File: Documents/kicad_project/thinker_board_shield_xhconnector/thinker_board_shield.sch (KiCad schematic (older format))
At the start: 10 parts, among them J1 Jack-DC, J2 Thinker_board_S, U1 XH_S, U2 1PIN, U3 XH_4PIN, U4 2_pin

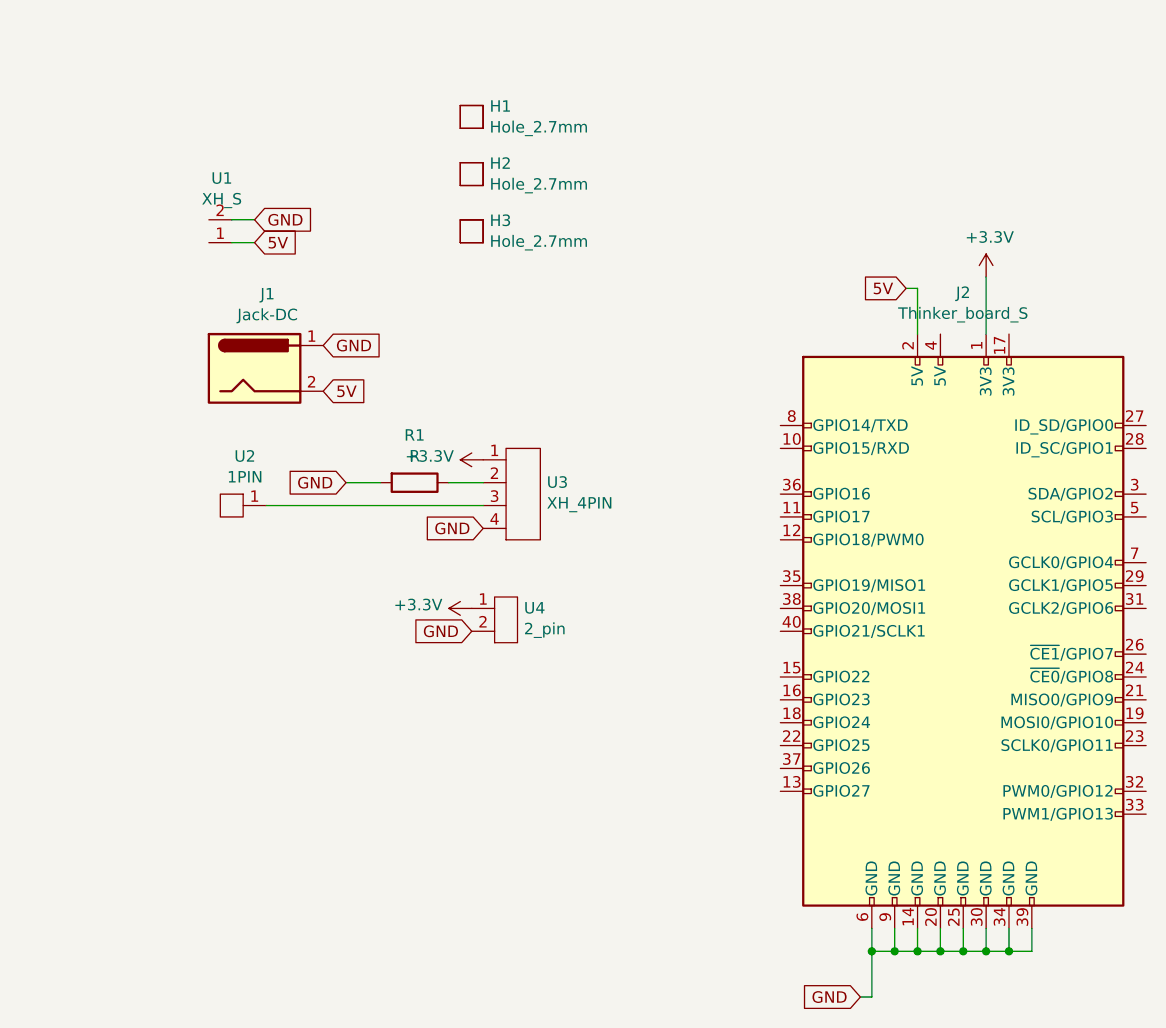
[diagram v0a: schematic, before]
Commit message: change to raspi
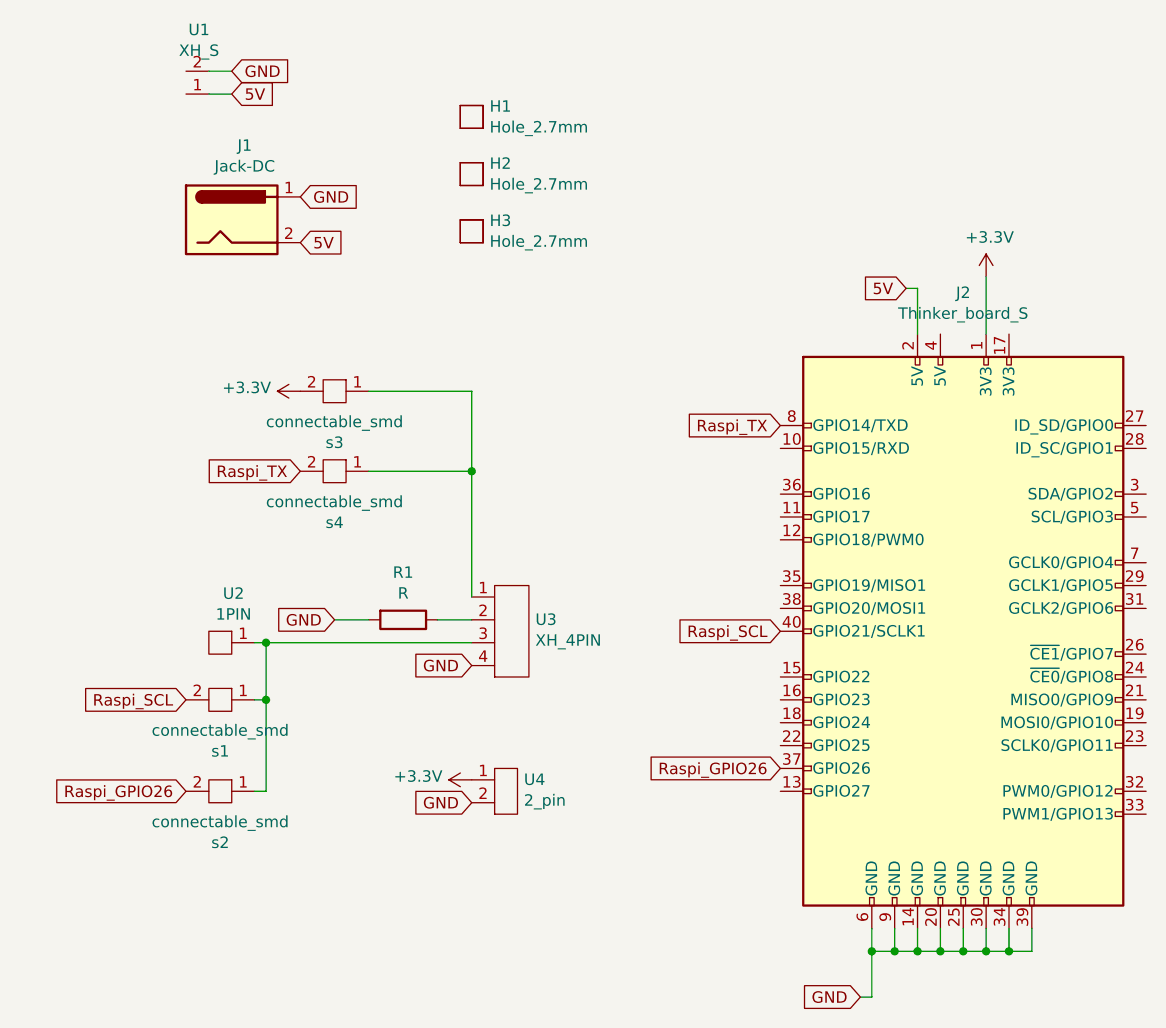
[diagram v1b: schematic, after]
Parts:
- added s1, s2, s3, s4: connectable_smd, hoshina_library:connectable_smd, symbol hoshina_library:connectable_smd
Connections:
- net +3V3: now also s3.2; no longer U3.1
- net Raspi_GPIO26: now reaches J2.37 (GPIO26)
- net Raspi_GPIO26: now also s2.2
- net Raspi_SCL: now reaches J2.40 (GPIO21/SCLK1)
- net Raspi_SCL: now also s1.2
- net Raspi_TX: now reaches J2.8 (GPIO14/TXD)
- net Raspi_TX: now also s4.2
- net at U2.1, U3.3: now also s1.1, s2.1
- new net: U3.1, s3.1, s4.1
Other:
- moved on the sheet: J1, R1, U1, U2, U3, U4
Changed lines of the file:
@@
 	1    0    0    -1
 $EndComp
-Text GLabel 1900 3450 2    50   Input ~ 0
+Text GLabel 1800 2800 2    50   Input ~ 0
 5V
-Text GLabel 1900 3250 2    50   Input ~ 0
+Text GLabel 1800 2600 2    50   Input ~ 0
 GND
 Text GLabel 4450 3000 0    50   Input ~ 0
@@
 Connection ~ 4900 5900
 Wire Wire Line
-	1500 2700 1600 2700
-Wire Wire Line
-	1600 2800 1500 2800
+	1400 2050 1500 2050
+Wire Wire Line
+	1500 2150 1400 2150
 $Comp
 L hoshina_library:XH_S U1
 U 1 1 5D710EE3
-P 1500 2700
-F 0 "U1" H 1543 2519 50  0000 C CNN
-F 1 "XH_S" H 1543 2610 50  0000 C CNN
-F 2 "hoshina_library:S2B-XH-A" H 1500 2600 50  0001 C CNN
-F 3 "" H 1500 2600 50  0001 C CNN
-	1    1500 2700
+P 1400 2050
+F 0 "U1" H 1443 1869 50  0000 C CNN
+F 1 "XH_S" H 1443 1960 50  0000 C CNN
+F 2 "hoshina_library:S2B-XH-A" H 1400 1950 50  0001 C CNN
+F 3 "" H 1400 1950 50  0001 C CNN
+	1    1400 2050
 	-1   0    0    1
 $EndComp
@@
 L hoshina_library:XH_4PIN U3
 U 1 1 5D76ADEE
-P 2600 3950
-F 0 "U3" H 2878 4051 50  0000 L CNN
-F 1 "XH_4PIN" H 2878 3960 50  0000 L CNN
-F 2 "hoshina_library:XH4PIN_S" H 2600 3750 50  0001 C CNN
-F 3 "" H 2600 3750 50  0001 C CNN
-	1    2600 3950
+P 2550 4550
+F 0 "U3" H 2828 4651 50  0000 L CNN
+F 1 "XH_4PIN" H 2828 4560 50  0000 L CNN
+F 2 "hoshina_library:XH4PIN_S" H 2550 4350 50  0001 C CNN
+F 3 "" H 2550 4350 50  0001 C CNN
+	1    2550 4550
 	1    0    0    -1
 $EndComp
@@
 L power:+3.3V #PWR0101
 U 1 1 5D76B7AA
-P 2600 3750
-F 0 "#PWR0101" H 2600 3600 50  0001 C CNN
-F 1 "+3.3V" V 2615 3878 50  0000 L CNN
-F 2 "" H 2600 3750 50  0001 C CNN
-F 3 "" H 2600 3750 50  0001 C CNN
-	1    2600 3750
+P 1800 3450
+F 0 "#PWR0101" H 1800 3300 50  0001 C CNN
+F 1 "+3.3V" V 1815 3578 50  0000 L CNN
+F 2 "" H 1800 3450 50  0001 C CNN
+F 3 "" H 1800 3450 50  0001 C CNN
+	1    1800 3450
 	0    -1   -1   0
 $EndComp
-Text GLabel 2000 3850 0    50   Input ~ 0
+Text GLabel 1950 4450 0    50   Input ~ 0
 GND
 $Comp
 L Device:R R1
 U 1 1 5D76C583
-P 2300 3850
-F 0 "R1" V 2093 3850 50  0000 C CNN
-F 1 "R" V 2184 3850 50  0000 C CNN
-F 2 "hoshina_library:register_0603" V 2230 3850 50  0001 C CNN
-F 3 "~" H 2300 3850 50  0001 C CNN
-	1    2300 3850
+P 2250 4450
+F 0 "R1" V 2043 4450 50  0000 C CNN
+F 1 "R" V 2134 4450 50  0000 C CNN
+F 2 "hoshina_library:register_0603" V 2180 4450 50  0001 C CNN
+F 3 "~" H 2250 4450 50  0001 C CNN
+	1    2250 4450
 	0    1    1    0
 $EndComp
 Wire Wire Line
-	2450 3850 2600 3850
-Wire Wire Line
-	2000 3850 2150 3850
-Text GLabel 2600 4050 0    50   Input ~ 0
+	2400 4450 2550 4450
+Wire Wire Line
+	1950 4450 2100 4450
+Text GLabel 2550 4650 0    50   Input ~ 0
 GND
 $Comp
 L hoshina_library:1PIN U2
 U 1 1 5D76DD85
-P 1650 3900
-F 0 "U2" H 1742 3735 50  0000 C CNN
-F 1 "1PIN" H 1742 3826 50  0000 C CNN
-F 2 "hoshina_library:1PIN" H 1750 3850 50  0001 C CNN
-F 3 "" H 1750 3850 50  0001 C CNN
-	1    1650 3900
-	-1   0    0    1
-$EndComp
-Wire Wire Line
-	2600 3950 1650 3950
+P 1600 4500
+F 0 "U2" H 1692 4335 50  0000 C CNN
+F 1 "1PIN" H 1692 4426 50  0000 C CNN
+F 2 "hoshina_library:1PIN" H 1700 4450 50  0001 C CNN
+F 3 "" H 1700 4450 50  0001 C CNN
+	1    1600 4500
+	-1   0    0    1
+$EndComp
+Wire Wire Line
+	2550 4550 1650 4550
 $Comp
 L power:+3.3V #PWR0102
@@
 L hoshina_library:2_pin U4
 U 1 1 5D790A94
-P 2650 4450
-F 0 "U4" H 2778 4501 50  0000 L CNN
-F 1 "2_pin" H 2778 4410 50  0000 L CNN
-F 2 "hoshina_library:2_pin" H 2650 4300 50  0001 C CNN
-F 3 "" H 2650 4300 50  0001 C CNN
-	1    2650 4450
-	1    0    0    -1
-$EndComp
-Text GLabel 2550 4500 0    50   Input ~ 0
+P 2650 5200
+F 0 "U4" H 2778 5251 50  0000 L CNN
+F 1 "2_pin" H 2778 5160 50  0000 L CNN
+F 2 "hoshina_library:2_pin" H 2650 5050 50  0001 C CNN
+F 3 "" H 2650 5050 50  0001 C CNN
+	1    2650 5200
+	1    0    0    -1
+$EndComp
+Text GLabel 2550 5250 0    50   Input ~ 0
 GND
 $Comp
 L power:+3.3V #PWR0103
 U 1 1 5D7912AC
-P 2550 4400
-F 0 "#PWR0103" H 2550 4250 50  0001 C CNN
-F 1 "+3.3V" V 2565 4528 50  0000 L CNN
-F 2 "" H 2550 4400 50  0001 C CNN
-F 3 "" H 2550 4400 50  0001 C CNN
-	1    2550 4400
+P 2550 5150
+F 0 "#PWR0103" H 2550 5000 50  0001 C CNN
+F 1 "+3.3V" V 2565 5278 50  0000 L CNN
+F 2 "" H 2550 5150 50  0001 C CNN
+F 3 "" H 2550 5150 50  0001 C CNN
+	1    2550 5150
 	0    -1   -1   0
 $EndComp
@@
 L Connector:Jack-DC J1
 U 1 1 5D792B55
-P 1600 3350
-F 0 "J1" H 1657 3675 50  0000 C CNN
-F 1 "Jack-DC" H 1657 3584 50  0000 C CNN
-F 2 "hoshina_library:DCJ" H 1650 3310 50  0001 C CNN
-F 3 "~" H 1650 3310 50  0001 C CNN
-	1    1600 3350
-	1    0    0    -1
-$EndComp
-Text GLabel 1600 2800 2    50   Input ~ 0
+P 1500 2700
+F 0 "J1" H 1557 3025 50  0000 C CNN
+F 1 "Jack-DC" H 1557 2934 50  0000 C CNN
+F 2 "hoshina_library:DCJ" H 1550 2660 50  0001 C CNN
+F 3 "~" H 1550 2660 50  0001 C CNN
+	1    1500 2700
+	1    0    0    -1
+$EndComp
+Text GLabel 1500 2150 2    50   Input ~ 0
 5V
-Text GLabel 1600 2700 2    50   Input ~ 0
-GND
+Text GLabel 1500 2050 2    50   Input ~ 0
+GND
+$Comp
+L hoshina_library:connectable_smd s3
+U 1 1 5D7B42C4
+P 1950 3450
+F 0 "s3" H 1950 3675 50  0000 C CNN
+F 1 "connectable_smd" H 1950 3584 50  0000 C CNN
+F 2 "hoshina_library:connectable_smd" H 1950 3300 50  0001 C CNN
+F 3 "" H 1950 3300 50  0001 C CNN
+	1    1950 3450
+	-1   0    0    1
+$EndComp
+$Comp
+L hoshina_library:connectable_smd s4
+U 1 1 5D7B9C1C
+P 1950 3800
+F 0 "s4" H 1950 4025 50  0000 C CNN
+F 1 "connectable_smd" H 1950 3934 50  0000 C CNN
+F 2 "hoshina_library:connectable_smd" H 1950 3650 50  0001 C CNN
+F 3 "" H 1950 3650 50  0001 C CNN
+	1    1950 3800
+	-1   0    0    1
+$EndComp
+Wire Wire Line
+	2100 3450 2550 3450
+Wire Wire Line
+	2550 3450 2550 3800
+Wire Wire Line
+	2100 3800 2550 3800
+Connection ~ 2550 3800
+Wire Wire Line
+	2550 3800 2550 4350
+Text GLabel 1800 3800 0    50   Input ~ 0
+Raspi_TX
+Text GLabel 3900 3600 0    50   Input ~ 0
+Raspi_TX
+$Comp
+L hoshina_library:connectable_smd s1
+U 1 1 5D7BBDD2
+P 1450 4800
+F 0 "s1" H 1450 5025 50  0000 C CNN
+F 1 "connectable_smd" H 1450 4934 50  0000 C CNN
+F 2 "hoshina_library:connectable_smd" H 1450 4650 50  0001 C CNN
+F 3 "" H 1450 4650 50  0001 C CNN
+	1    1450 4800
+	-1   0    0    1
+$EndComp
+Text GLabel 1300 4800 0    50   Input ~ 0
+Raspi_SCL
+$Comp
+L hoshina_library:connectable_smd s2
+U 1 1 5D7BCB7C
+P 1450 5200
+F 0 "s2" H 1450 5425 50  0000 C CNN
+F 1 "connectable_smd" H 1450 5334 50  0000 C CNN
+F 2 "hoshina_library:connectable_smd" H 1450 5050 50  0001 C CNN
+F 3 "" H 1450 5050 50  0001 C CNN
+	1    1450 5200
+	-1   0    0    1
+$EndComp
+Text GLabel 1300 5200 0    50   Input ~ 0
+Raspi_GPIO26
+Wire Wire Line
+	1600 4800 1650 4800
+Wire Wire Line
+	1650 4800 1650 4550
+Connection ~ 1650 4550
+Wire Wire Line
+	1650 4550 1600 4550
+Wire Wire Line
+	1650 4800 1650 5200
+Wire Wire Line
+	1650 5200 1600 5200
+Connection ~ 1650 4800
+Text GLabel 3900 4500 0    50   Input ~ 0
+Raspi_SCL
+Text GLabel 3900 5100 0    50   Input ~ 0
+Raspi_GPIO26
 $EndSCHEMATC
